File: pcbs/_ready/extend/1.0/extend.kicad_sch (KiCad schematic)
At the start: 25 parts, among them J1 Conn_01x02_Male, J10 Conn_01x02_Male, J11 Conn_01x02_Pin, J12 Conn_01x03_Pin, J2 Conn_01x05_Pin, J3 Conn_01x04_Pin, J4 Conn_01x06_Pin, J5 Conn_01x02_Male, J6 Conn_01x02_Male, J7 Conn_01x04_Pin, J8 Conn_01x05_Pin, J9 Conn_01x02_Pin, U1 MCP23017_SS

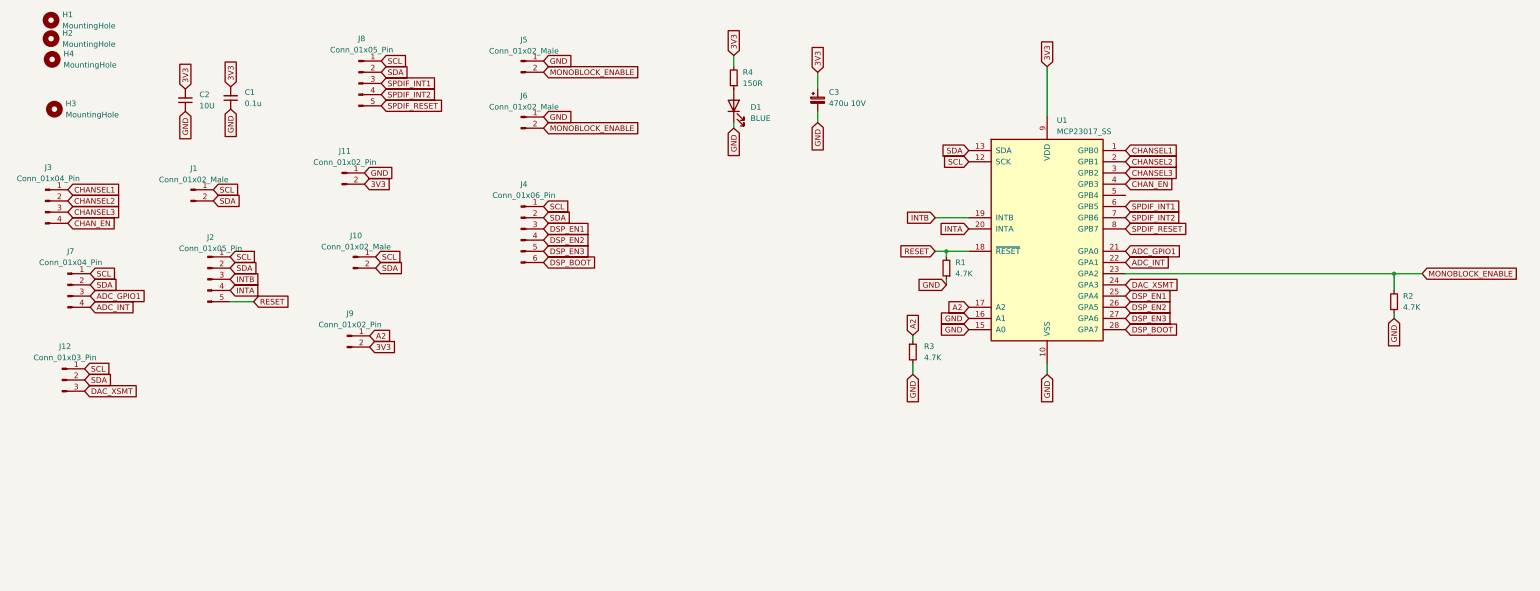
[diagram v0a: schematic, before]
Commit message: Updates
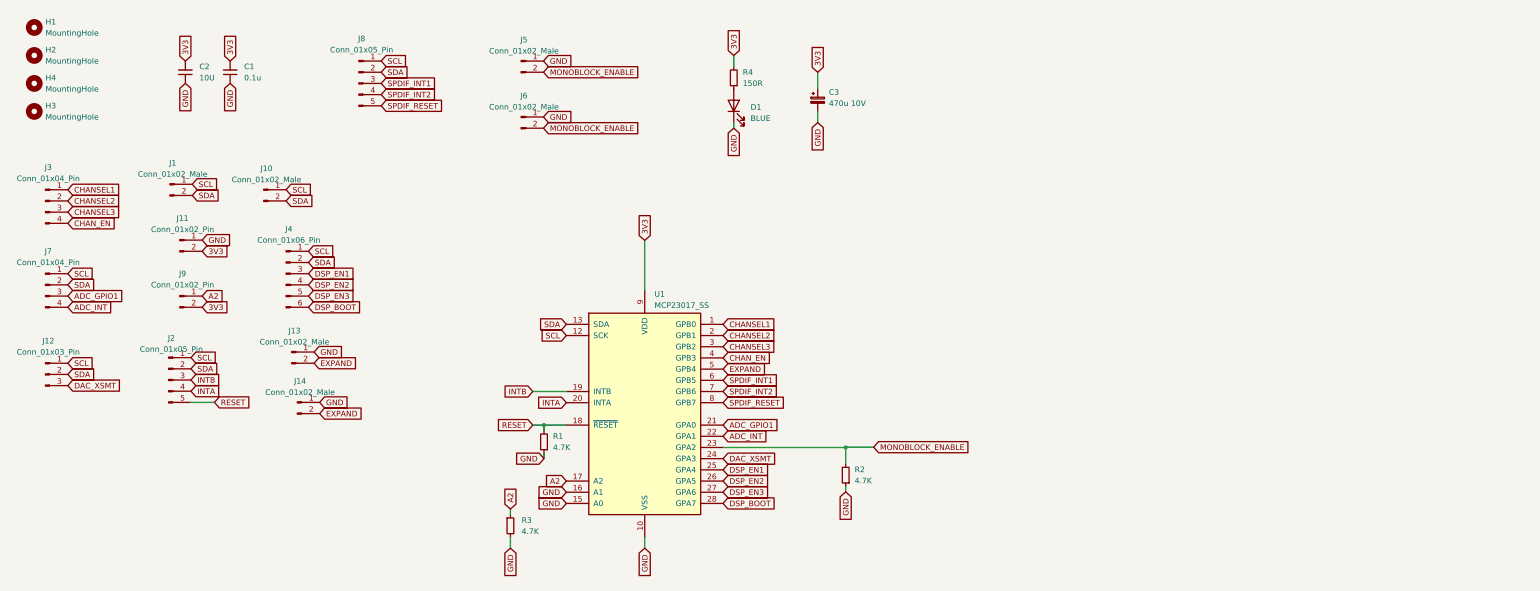
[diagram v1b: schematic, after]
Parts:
- added J13: Conn_01x02_Male, Connector_JST:JST_PH_B2B-PH-K_1x02_P2.00mm_Vertical, symbol Connector:Conn_01x02_Male
- added J14: Conn_01x02_Male, Connector_PinHeader_2.54mm:PinHeader_1x02_P2.54mm_Vertical, symbol Connector:Conn_01x02_Male
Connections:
- net GND: now also J13.1 (Pin_1), J14.1 (Pin_1)
- net EXPAND: now reaches U1.5 (GPB4)
- net EXPAND: now also J13.2 (Pin_2), J14.2 (Pin_2)
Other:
- moved on the sheet: C1, C2, H1, H2, H3, H4, J1, J10, J11, J12, J2, J4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
